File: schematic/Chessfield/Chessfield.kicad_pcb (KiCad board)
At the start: 2 copper layers, 35 x 35 mm, 13 parts, among them J1 Conn_01x04_Pin, J2 Conn_01x04_Pin, J3 Conn_01x04_Pin, J4 Conn_01x04_Pin

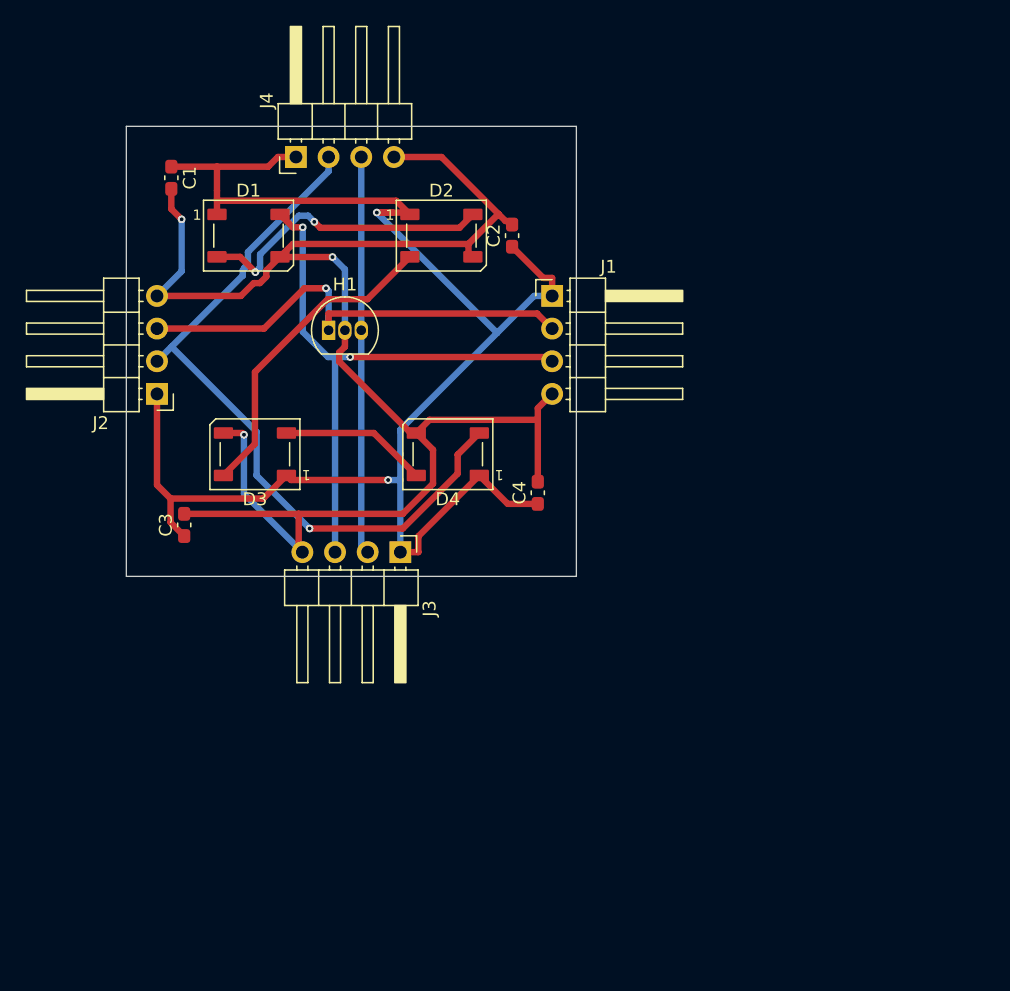
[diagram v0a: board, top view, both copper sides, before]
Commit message: finish chessfield
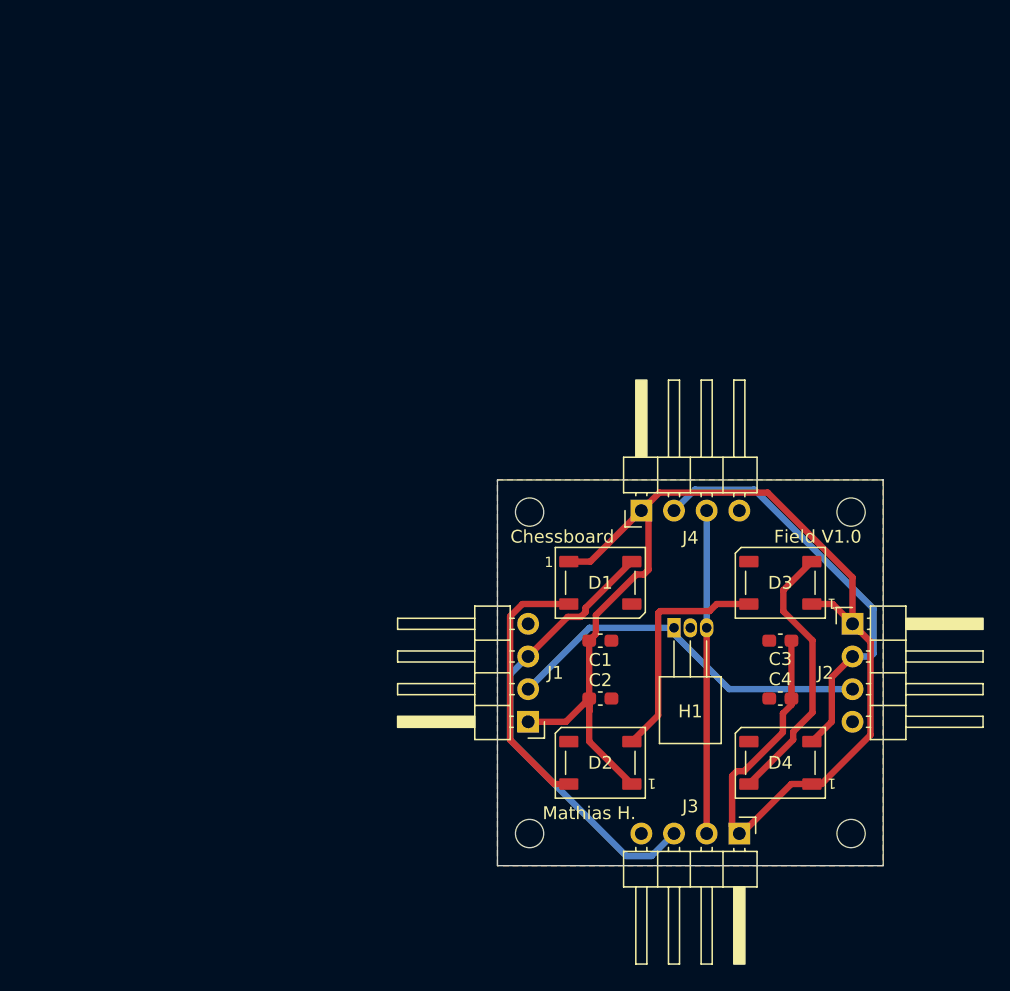
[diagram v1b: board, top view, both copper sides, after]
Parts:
- added REF**: MountingHole_2.2mm_M2, MountingHole:MountingHole_2.2mm_M2, F.Cu at (133.4, 108.0)
- added REF**: MountingHole_2.2mm_M2, MountingHole:MountingHole_2.2mm_M2, F.Cu at (133.4, 83.0)
- added REF**: MountingHole_2.2mm_M2, MountingHole:MountingHole_2.2mm_M2, F.Cu at (158.4, 108.0)
- added REF**: MountingHole_2.2mm_M2, MountingHole:MountingHole_2.2mm_M2, F.Cu at (158.4, 83.0)
- H1: footprint Package_TO_SOT_THT:TO-92_Inline -> Package_TO_SOT_THT:TO-92_Inline_Horizontal1
- moved J2 57.0 mm to (158.5, 91.7), turned to 0 degrees
- moved C1 49.1 mm to (138.9, 93.0), turned to 0 degrees
- moved C3 47.2 mm to (152.9, 93.0), turned to 180 degrees
- moved D2 42.8 mm to (138.9, 102.5), turned to 180 degrees
- moved D3 42.1 mm to (152.9, 88.5)
- moved J4 38.4 mm to (142.1, 82.9)
- moved D1 38.4 mm to (138.9, 88.5)
- moved C2 36.6 mm to (138.9, 97.5), turned to 0 degrees
- moved H1 35.5 mm to (144.6, 92.0)
- moved D4 35.3 mm to (152.9, 102.5)
- moved J3 34.3 mm to (149.7, 108.0)
- moved J1 33.2 mm to (133.2, 99.3), turned to 180 degrees
- moved C4 24.7 mm to (152.9, 97.5), turned to 180 degrees
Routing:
- net GND: track 130.3 -> 0.00 mm, vias 3 -> 0
- net DOL: track 57.1 -> 33.2 mm, vias 1 -> 0
- net +5V: track 126.5 -> 106.3 mm, vias 2 -> 0
- net DIL: track 45.8 -> 35.6 mm, vias 2 -> 0
- net Net-(D3-DOUT): track 11.5 -> 21.2 mm
- net VS: track 37.0 -> 29.5 mm, vias 1 -> 0
- net Net-(D2-DOUT): track 24.8 -> 18.2 mm
- net DOS: track 30.9 -> 25.6 mm
- net Net-(D1-DOUT): track 23.6 -> 20.6 mm, vias 2 -> 0
- added copper zone on B.Cu, net GND
- added copper zone on F.Cu, net GND
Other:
- board size 35 x 35 mm -> 30 x 30 mm
- board text added: "Chessboard"
- board text added: "Field V1.0"
- board text added: "Mathias H."
